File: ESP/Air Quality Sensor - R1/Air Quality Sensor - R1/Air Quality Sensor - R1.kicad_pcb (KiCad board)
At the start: 2 copper layers, 101.6 x 76.2 mm, 27 parts, among them U1 SCD4X, U2 CCS811, U3 SGP40, U4 Sensair_Sunrise_006-0-0007, U5 MICS-VZ-89TE‎, U6 SCD30, U7 BME680

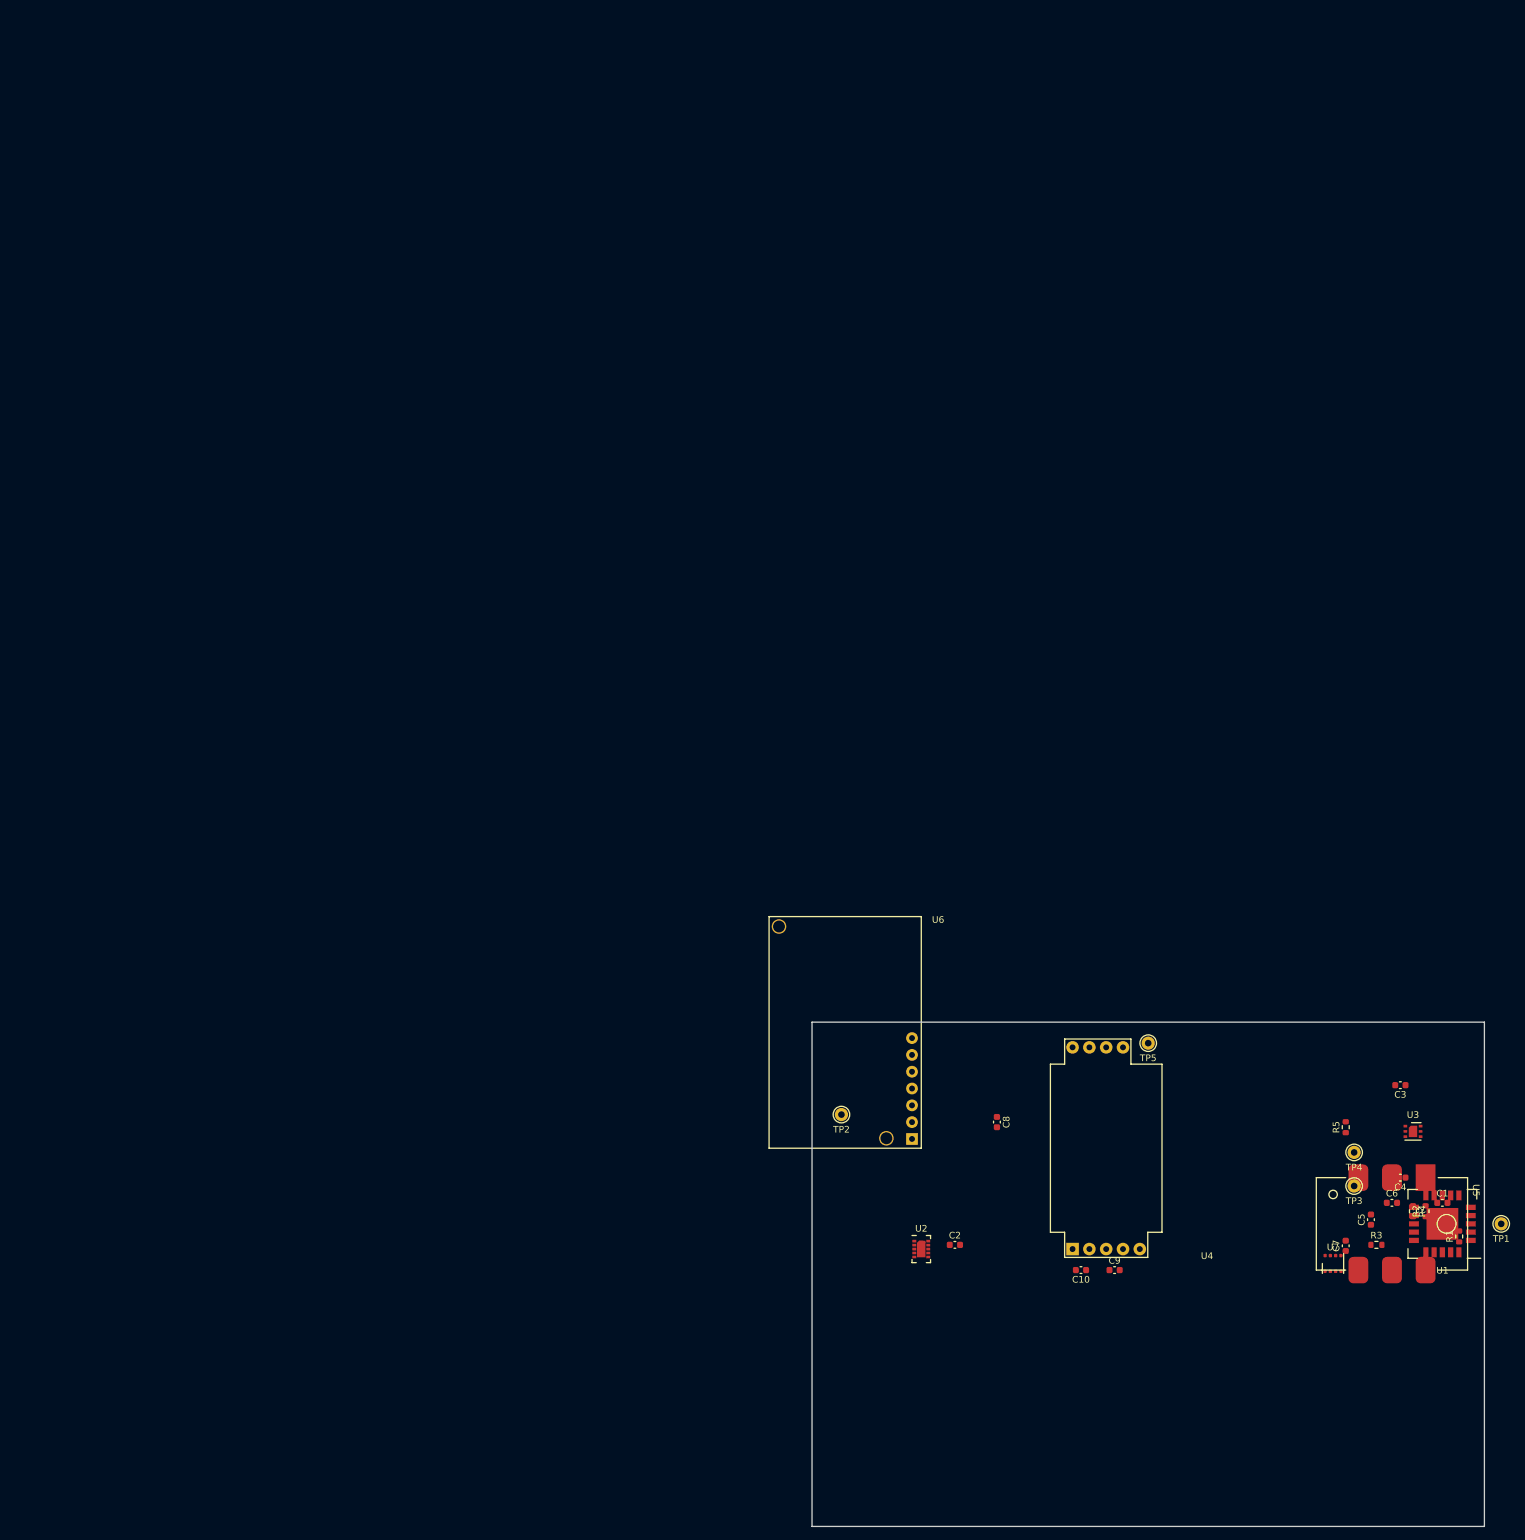
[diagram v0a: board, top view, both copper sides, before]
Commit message: Pile of uncommitted boards.
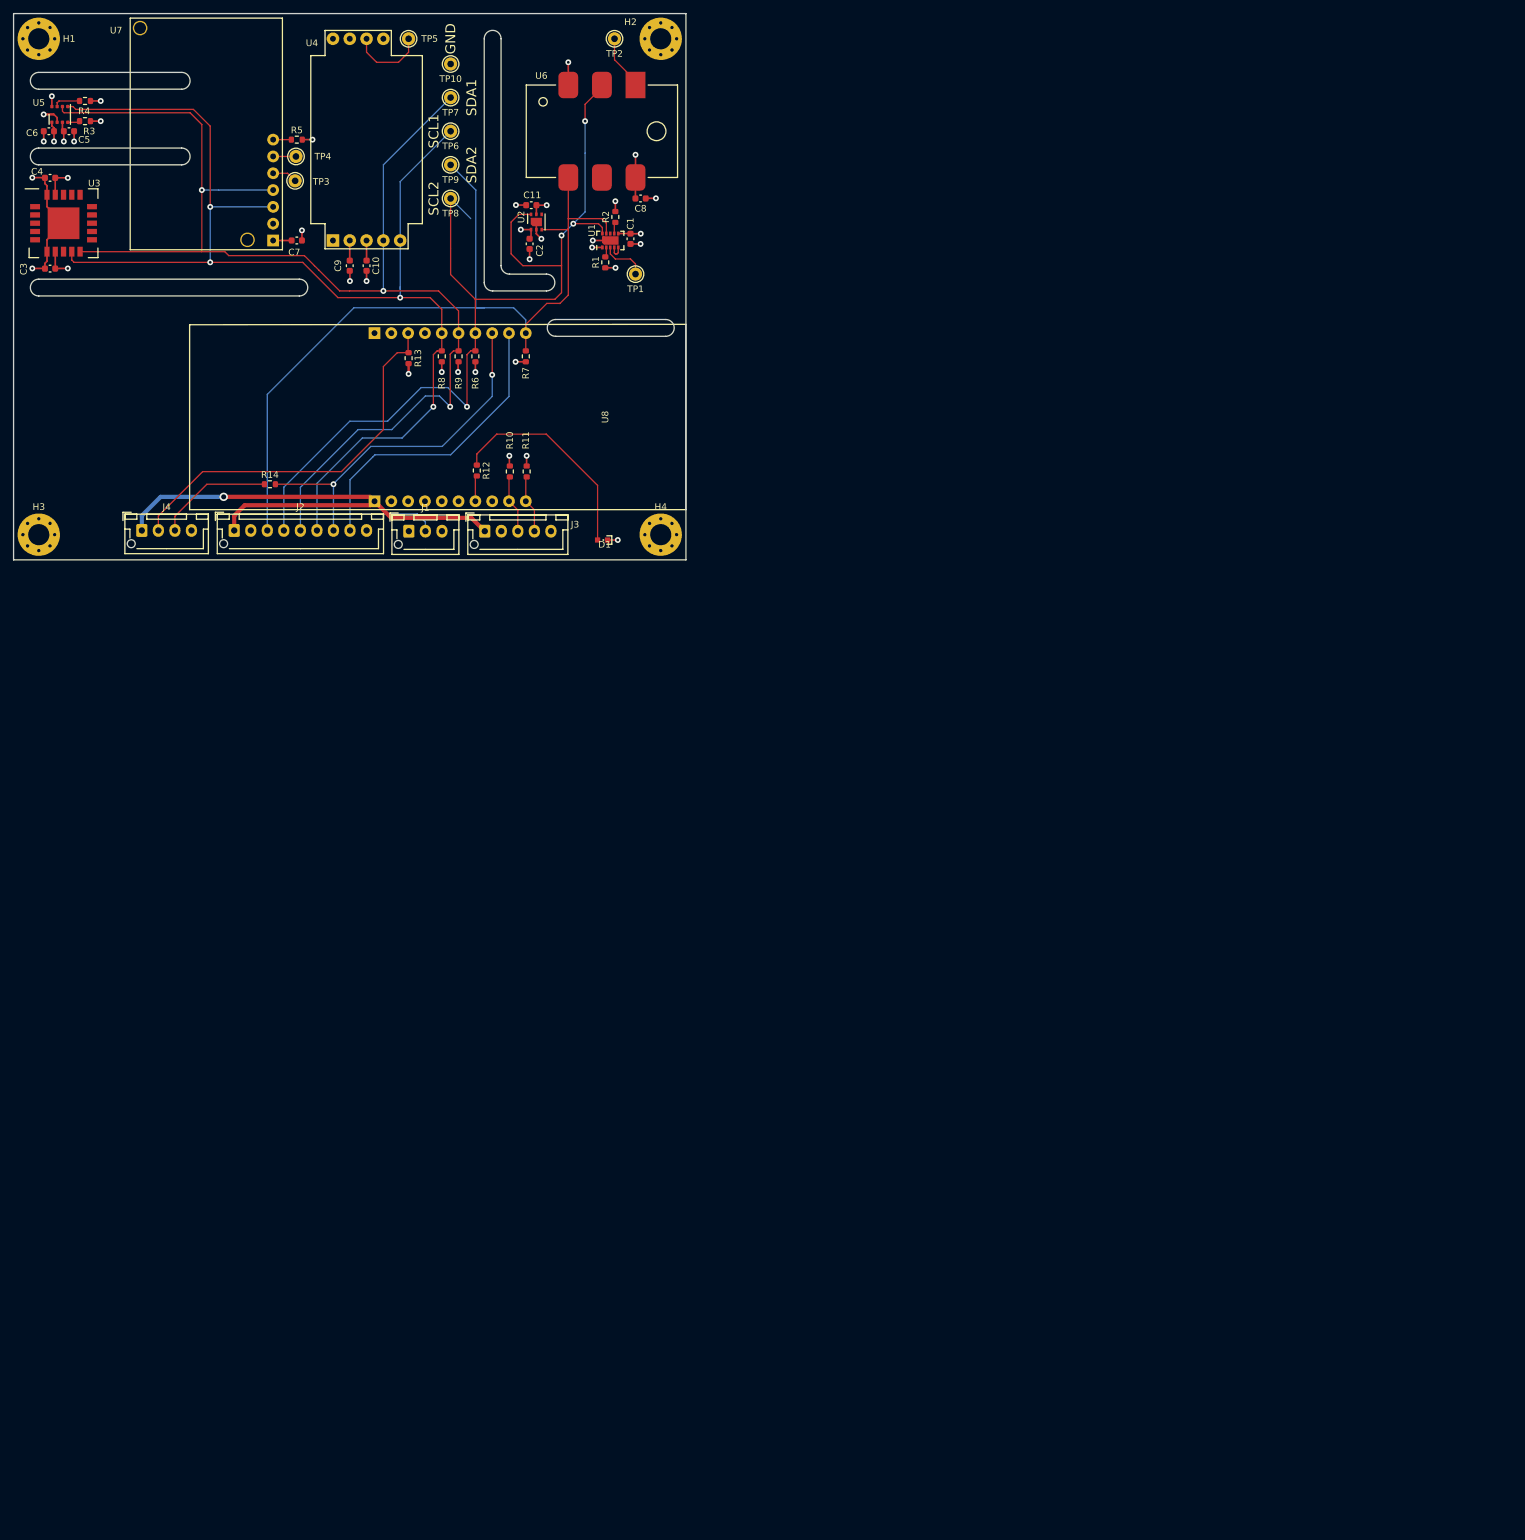
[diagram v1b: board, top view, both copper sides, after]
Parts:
- added C11: 0.1u, Capacitor_SMD:C_0603_1608Metric, F.Cu at (78.2, -53.6)
- added D1: LED, custom:CHIPLED_0603, F.Cu at (89.0, -3.00)
- added H1: MountingHole, MountingHole:MountingHole_3.2mm_M3_Pad_Via, F.Cu at (3.81, -78.7)
- added H2: MountingHole, MountingHole:MountingHole_3.2mm_M3_Pad_Via, F.Cu at (97.8, -78.7)
- added H3: MountingHole, MountingHole:MountingHole_3.2mm_M3_Pad_Via, F.Cu at (3.81, -3.81)
- added H4: MountingHole, MountingHole:MountingHole_3.2mm_M3_Pad_Via, F.Cu at (97.8, -3.81)
- added J1: Conn_01x05, Connector_JST:JST_XH_B3B-XH-AM_1x03_P2.50mm_Vertical, F.Cu at (59.7, -4.33)
- added J2: Conn_01x09, Connector_JST:JST_XH_B9B-XH-AM_1x09_P2.50mm_Vertical, F.Cu at (33.3, -4.45)
- added J3: Conn_01x05, Connector_JST:JST_XH_B5B-XH-AM_1x05_P2.50mm_Vertical, F.Cu at (71.2, -4.33)
- added J4: Conn_01x04, Connector_JST:JST_XH_B4B-XH-AM_1x04_P2.50mm_Vertical, F.Cu at (19.4, -4.45)
- added R10: 4.7K, Resistor_SMD:R_0603_1608Metric, F.Cu at (75.0, -13.4)
- added R11: 4.7K, Resistor_SMD:R_0603_1608Metric, F.Cu at (77.5, -13.4)
- added R12: 470R, Resistor_SMD:R_0603_1608Metric, F.Cu at (70.0, -13.5)
- added R13: 4.7K, Resistor_SMD:R_0603_1608Metric, F.Cu at (59.7, -30.5)
- added R14: 470R, Resistor_SMD:R_0603_1608Metric, F.Cu at (38.7, -11.4)
- added R6: 4.7K, Resistor_SMD:R_0603_1608Metric, F.Cu at (69.8, -30.8)
- added R7: 4.7K, Resistor_SMD:R_0603_1608Metric, F.Cu at (77.4, -30.8)
- added R8: 4.7K, Resistor_SMD:R_0603_1608Metric, F.Cu at (64.7, -30.8)
- added R9: 4.7K, Resistor_SMD:R_0603_1608Metric, F.Cu at (67.2, -30.8)
- added TP10: TestPoint_Small, Connector_Pin:Pin_D1.0mm_L10.0mm, F.Cu at (66.0, -74.9)
- added TP6: TestPoint_Small, Connector_Pin:Pin_D1.0mm_L10.0mm, F.Cu at (66.0, -64.8)
- added TP7: TestPoint_Small, Connector_Pin:Pin_D1.0mm_L10.0mm, F.Cu at (66.0, -69.8)
- added TP8: TestPoint_Small, Connector_Pin:Pin_D1.0mm_L10.0mm, F.Cu at (66.0, -54.6)
- added TP9: TestPoint_Small, Connector_Pin:Pin_D1.0mm_L10.0mm, F.Cu at (66.0, -59.7)
- added U8: ESP32-POE, custom:ESP32-POE, F.Cu at (101.6, -21.6)
- C2, C7: value 0.1u -> 1.0u
- C4, C9: value 1.0u -> 0.1u
- U1: value SCD4X -> CCS811; footprint Sensor_Gas:Sensirion_SCD4X_QFN-20_EP_10.1x10.1_Pitch1.25mm -> Package_LGA:AMS_LGA-10-1EP_2.7x4mm_P0.6mm
- U2: value CCS811 -> SGP40; footprint Package_LGA:AMS_LGA-10-1EP_2.7x4mm_P0.6mm -> Sensor_Gas:Sensirion_DFN-6-1EP_2.44x2.44mm_P0.8mm
- U3: value SGP40 -> SCD4X; footprint Sensor_Gas:Sensirion_DFN-6-1EP_2.44x2.44mm_P0.8mm -> Sensor_Gas:Sensirion_SCD4X_QFN-20_EP_10.1x10.1_Pitch1.25mm
- U5: value MICS-VZ-89TE‎ -> BME680; footprint Sensor_Gas:Telaire_MICS-VZ-89TE‎ -> Package_LGA:Bosch_LGA-8_3x3mm_P0.8mm_ClockwisePinNumbering
- U6: value SCD30 -> MICS-VZ-89TE‎; footprint Sensor_Gas:Sensiron_SCD30_Module -> Sensor_Gas:Telaire_MICS-VZ-89TE‎
- U7: value BME680 -> SCD30; footprint Package_LGA:Bosch_LGA-8_3x3mm_P0.8mm_ClockwisePinNumbering -> Sensor_Gas:Sensiron_SCD30_Module
- moved U5 262.0 mm to (6.99, -67.3), turned to 0 degrees
- moved R4 261.6 mm to (10.8, -69.3), turned to 180 degrees
- moved C6 259.6 mm to (5.33, -64.8), turned to 180 degrees
- moved R3 258.7 mm to (10.8, -66.3), turned to 180 degrees
- moved C5 256.4 mm to (8.37, -64.8), turned to 0 degrees
- moved C4 253.9 mm to (5.52, -57.7)
- moved U3 245.8 mm to (7.55, -50.9)
- moved C3 238.4 mm to (5.52, -44.0)
- moved TP3 220.6 mm to (42.5, -57.3)
- moved U7 220.6 mm to (40.6, -46.9)
- moved TP4 219.6 mm to (42.7, -61.0)
- moved C7 219.5 mm to (42.8, -48.3), turned to 0 degrees
- moved R5 217.7 mm to (42.8, -63.5), turned to 0 degrees
- moved R1 195.7 mm to (89.4, -45.0)
- moved U1 194.6 mm to (90.2, -48.3), turned to 90 degrees
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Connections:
- U1 pad 1: (no net) -> GND
- U1 pad 10: /SENS/SDA -> /SENS/SCL_2
- U1 pad 11: (no net) -> GND
- U1 pad 2: (no net) -> Net-(R1-Pad2)
- U1 pad 3: (no net) -> Net-(TP1-Pad1)
- U1 pad 4: (no net) -> Net-(U1-Pad4)
- U1 pad 5: (no net) -> Net-(U1-Pad4)
- U1 pad 6: GND -> +3V3
- U1 pad 7: +3V3 -> Net-(R2-Pad1)
- U1 pad 8: (no net) -> unconnected-(U1-Pad8)
- U1 pad 9: /SENS/SCL -> /SENS/SDA_2
- U2 pad 1: GND -> +3V3
- U2 pad 2: Net-(R1-Pad2) -> GND
- U2 pad 3: Net-(TP1-Pad1) -> /SENS/SDA_2
- U2 pad 4: Net-(U2-Pad4) -> unconnected-(U2-Pad4)
- U2 pad 5: Net-(U2-Pad4) -> +3V3
- U2 pad 6: +3V3 -> /SENS/SCL_2
- U2 pad 7: Net-(R2-Pad1) -> GND
- U3 pad 1: +3V3 -> (no net)
- U3 pad 2: GND -> (no net)
- U3 pad 3: /SENS/SDA -> (no net)
- U3 pad 4: unconnected-(U3-Pad4) -> (no net)
- U3 pad 5: +3V3 -> (no net)
- U3 pad 6: /SENS/SCL -> GND
- U3 pad 7: GND -> +3V3
- U4 pad 4: /SENS/SDA -> /SENS/SDA_1
- U4 pad 5: /SENS/SCL -> /SENS/SCL_1
- U4 pad 7: Net-(TP2-Pad1) -> Net-(TP5-Pad1)
- U5 pad 1: Net-(TP3-Pad1) -> GND
- U5 pad 2: /SENS/SCL -> Net-(R4-Pad2)
- U5 pad 3: GND -> /SENS/SDA_1
- U5 pad 4: /SENS/SDA -> /SENS/SCL_1
- U5 pad 5: unconnected-(U5-Pad5) -> Net-(R3-Pad2)
- U6 pad 1: +3V3 -> Net-(TP2-Pad1)
- U6 pad 2: GND -> /SENS/SCL_2
- U6 pad 3: /SENS/SCL -> GND
- U6 pad 4: /SENS/SDA -> /SENS/SDA_2
- U6 pad 5: Net-(TP4-Pad1) -> unconnected-(U6-Pad5)
- U6 pad 6: Net-(TP5-Pad1) -> +3V3
- U7 pad 1: GND -> +3V3
- U7 pad 2: Net-(R4-Pad2) -> GND
- U7 pad 3: /SENS/SDA -> /SENS/SCL_1
- U7 pad 4: /SENS/SCL -> /SENS/SDA_1
- U7 pad 5: Net-(R3-Pad2) -> Net-(TP3-Pad1)
- U7 pad 6: +3V3 -> Net-(TP4-Pad1)
- U7 pad 7: GND -> Net-(R5-Pad1)
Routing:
- net /SENS/SDA_1: track 0.00 -> 197.9 mm, vias 0 -> 3
- net /SENS/SCL_1: track 0.00 -> 186.9 mm, vias 0 -> 4
- net /SENS/SCL_2: track 0.00 -> 149.5 mm, vias 0 -> 4
- net /SENS/SDA_2: track 0.00 -> 134.1 mm
- net +5V: track 0.00 -> 81.7 mm, vias 0 -> 1
- net GND: track 0.00 -> 65.4 mm, vias 0 -> 20
- net Net-(J1-Pad2): track 0.00 -> 59.7 mm
- net Net-(R13-Pad1): track 0.00 -> 58.8 mm
- net +3V3: track 0.00 -> 55.3 mm, vias 0 -> 18
- net Net-(J2-Pad7): track 0.00 -> 54.8 mm, vias 0 -> 2
- net Net-(D1-Pad2): track 0.00 -> 32.6 mm
- net Net-(R14-Pad1): track 0.00 -> 17.7 mm
- net Net-(TP5-Pad1): track 0.00 -> 11.7 mm
- net Net-(J3-Pad3): track 0.00 -> 8.81 mm
- net Net-(J3-Pad4): track 0.00 -> 8.79 mm
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- added copper zone on In2.Cu, net +3V3
- added copper zone on In1.Cu, net GND
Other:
- board size 101.6 x 76.2 mm -> 101.6 x 82.5 mm
- copper layers 2 -> 4
- board text added: "GND"
- board text added: "SCL1"
- board text added: "SCL2"
- board text added: "SDA1"
- board text added: "SDA2"
